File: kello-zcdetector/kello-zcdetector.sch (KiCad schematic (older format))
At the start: 8 parts, among them J1 Conn_01x02_Male, J2 Conn_01x02_Male, U1 LTV-817S

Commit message: joo
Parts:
- R1, R2, R3, R4: footprint Resistor_SMD:R_1206_3216Metric -> Resistor_SMD:R_0805_2012Metric
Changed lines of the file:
@@
 F 0 "R1" V 1893 3150 50  0000 C CNN
 F 1 "100k" V 1984 3150 50  0000 C CNN
-F 2 "Resistor_SMD:R_1206_3216Metric" V 2030 3150 50  0001 C CNN
+F 2 "Resistor_SMD:R_0805_2012Metric" V 2030 3150 50  0001 C CNN
 F 3 "~" H 2100 3150 50  0001 C CNN
 	1    2100 3150
@@
 F 0 "R2" V 1893 3500 50  0000 C CNN
 F 1 "100k" V 1984 3500 50  0000 C CNN
-F 2 "Resistor_SMD:R_1206_3216Metric" V 2030 3500 50  0001 C CNN
+F 2 "Resistor_SMD:R_0805_2012Metric" V 2030 3500 50  0001 C CNN
 F 3 "~" H 2100 3500 50  0001 C CNN
 	1    2100 3500
@@
 F 0 "R3" V 2393 3150 50  0000 C CNN
 F 1 "100k" V 2484 3150 50  0000 C CNN
-F 2 "Resistor_SMD:R_1206_3216Metric" V 2530 3150 50  0001 C CNN
+F 2 "Resistor_SMD:R_0805_2012Metric" V 2530 3150 50  0001 C CNN
 F 3 "~" H 2600 3150 50  0001 C CNN
 	1    2600 3150
@@
 F 0 "R4" V 2393 3500 50  0000 C CNN
 F 1 "100k" V 2484 3500 50  0000 C CNN
-F 2 "Resistor_SMD:R_1206_3216Metric" V 2530 3500 50  0001 C CNN
+F 2 "Resistor_SMD:R_0805_2012Metric" V 2530 3500 50  0001 C CNN
 F 3 "~" H 2600 3500 50  0001 C CNN
 	1    2600 3500

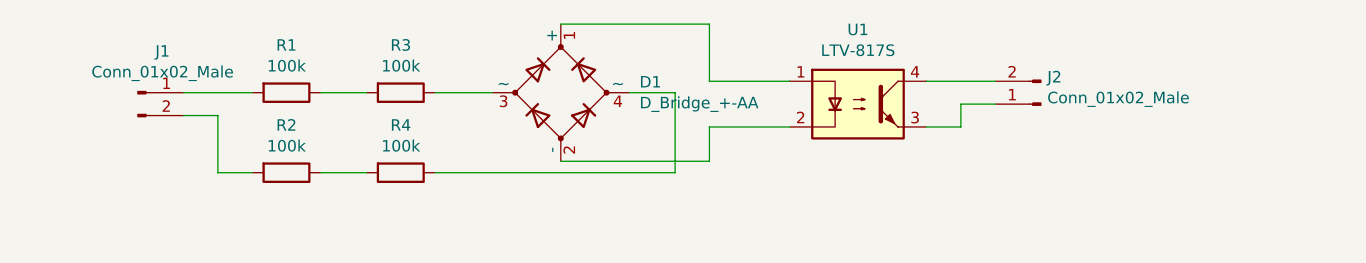
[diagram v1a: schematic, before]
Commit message: joo
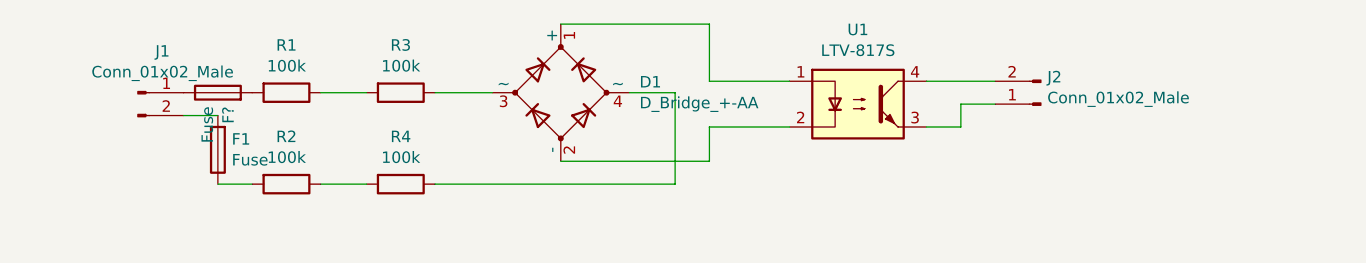
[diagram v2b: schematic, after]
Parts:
- added F1, F?: Fuse, Fuse:Fuse_10mmx3mm, symbol Device:Fuse
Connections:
- net at R1.2: now also F?.2; no longer J1.1 (Pin_1)
- net at R2.2: now also F1.1; no longer J1.2 (Pin_2)
- new net: F1.2, J1.2 (Pin_2)
- new net: F?.1, J1.1 (Pin_1)
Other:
- moved on the sheet: R2, R4
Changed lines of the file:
@@
 L Device:R R2
 U 1 1 5E892730
-P 2100 3500
-F 0 "R2" V 1893 3500 50  0000 C CNN
-F 1 "100k" V 1984 3500 50  0000 C CNN
-F 2 "Resistor_SMD:R_0805_2012Metric" V 2030 3500 50  0001 C CNN
-F 3 "~" H 2100 3500 50  0001 C CNN
-	1    2100 3500
+P 2100 3550
+F 0 "R2" V 1893 3550 50  0000 C CNN
+F 1 "100k" V 1984 3550 50  0000 C CNN
+F 2 "Resistor_SMD:R_0805_2012Metric" V 2030 3550 50  0001 C CNN
+F 3 "~" H 2100 3550 50  0001 C CNN
+	1    2100 3550
 	0    1    1    0
 $EndComp
@@
 L Device:R R4
 U 1 1 5E8929D6
-P 2600 3500
-F 0 "R4" V 2393 3500 50  0000 C CNN
-F 1 "100k" V 2484 3500 50  0000 C CNN
-F 2 "Resistor_SMD:R_0805_2012Metric" V 2530 3500 50  0001 C CNN
-F 3 "~" H 2600 3500 50  0001 C CNN
-	1    2600 3500
+P 2600 3550
+F 0 "R4" V 2393 3550 50  0000 C CNN
+F 1 "100k" V 2484 3550 50  0000 C CNN
+F 2 "Resistor_SMD:R_0805_2012Metric" V 2530 3550 50  0001 C CNN
+F 3 "~" H 2600 3550 50  0001 C CNN
+	1    2600 3550
 	0    1    1    0
 $EndComp
@@
 $EndComp
 Wire Wire Line
-	1650 3150 1950 3150
-Wire Wire Line
 	1650 3250 1800 3250
 Wire Wire Line
-	1800 3250 1800 3500
-Wire Wire Line
-	1800 3500 1950 3500
-Wire Wire Line
-	2250 3500 2450 3500
+	2250 3550 2450 3550
 Wire Wire Line
 	2250 3150 2450 3150
@@
 	3000 3150 2750 3150
 Wire Wire Line
-	2750 3500 3800 3500
-Wire Wire Line
-	3800 3500 3800 3150
+	2750 3550 3800 3550
 Wire Wire Line
 	3800 3150 3600 3150
@@
 Wire Wire Line
 	5050 3200 5200 3200
+$Comp
+L Device:Fuse F1
+U 1 1 5E4EBF45
+P 1800 3400
+F 0 "F1" H 1740 3354 50  0000 R CNN
+F 1 "Fuse" H 1740 3445 50  0000 R CNN
+F 2 "Fuse:Fuse_10mmx3mm" V 1730 3400 50  0001 C CNN
+F 3 "~" H 1800 3400 50  0001 C CNN
+	1    1800 3400
+	-1   0    0    1
+$EndComp
+Wire Wire Line
+	3800 3150 3800 3550
+Wire Wire Line
+	1800 3550 1950 3550
+$Comp
+L Device:Fuse F?
+U 1 1 5EDDD343
+P 1800 3150
+F 0 "F?" H 1740 3104 50  0000 R CNN
+F 1 "Fuse" H 1740 3195 50  0000 R CNN
+F 2 "Fuse:Fuse_10mmx3mm" V 1730 3150 50  0001 C CNN
+F 3 "~" H 1800 3150 50  0001 C CNN
+	1    1800 3150
+	0    -1   -1   0
+$EndComp
 $EndSCHEMATC

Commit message: diodisillalla zcdet
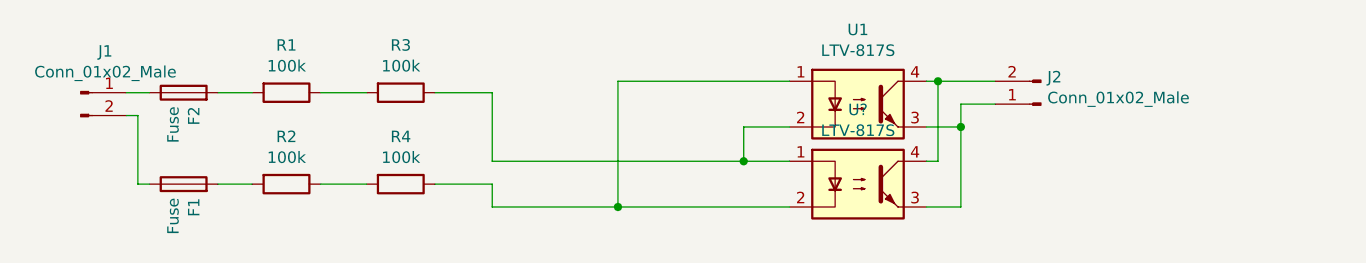
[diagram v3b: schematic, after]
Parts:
- removed D1: D_Bridge_+-AA, Diode_SMD:Diode_Bridge_Diotec_SO-DIL-Slim, symbol Device:D_Bridge_+-AA
- added U?: LTV-817S, Package_DIP:SMDIP-4_W9.53mm, symbol Isolator:LTV-817S
- gave numbers to parts that had none: 1
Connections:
- net at F1.1: now also J1.2 (Pin_2); no longer R2.2
- net at F1.2: now also R2.2; no longer J1.2 (Pin_2)
- net at R3.1: now also U1.2, U?.1
- net at R4.1: now also U1.1, U?.2
- net at J2.1 (Pin_1), U1.3: now also U?.3
- net at J2.2 (Pin_2), U1.4: now also U?.4
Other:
- moved on the sheet: F1, F2, J1
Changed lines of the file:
@@
 L Connector:Conn_01x02_Male J1
 U 1 1 5E892E28
-P 1450 3150
-F 0 "J1" H 1558 3331 50  0000 C CNN
-F 1 "Conn_01x02_Male" H 1558 3240 50  0000 C CNN
-F 2 "Connector_PinHeader_2.54mm:PinHeader_1x02_P2.54mm_Vertical" H 1450 3150 50  0001 C CNN
-F 3 "~" H 1450 3150 50  0001 C CNN
-	1    1450 3150
+P 1200 3150
+F 0 "J1" H 1308 3331 50  0000 C CNN
+F 1 "Conn_01x02_Male" H 1308 3240 50  0000 C CNN
+F 2 "Connector_PinHeader_2.54mm:PinHeader_1x02_P2.54mm_Vertical" H 1200 3150 50  0001 C CNN
+F 3 "~" H 1200 3150 50  0001 C CNN
+	1    1200 3150
 	1    0    0    -1
 $EndComp
-Wire Wire Line
-	1650 3250 1800 3250
 Wire Wire Line
 	2250 3550 2450 3550
 Wire Wire Line
 	2250 3150 2450 3150
-$Comp
-L Device:D_Bridge_+-AA D1
-U 1 1 5E893821
-P 3300 3150
-F 0 "D1" V 3346 2806 50  0000 R CNN
-F 1 "D_Bridge_+-AA" V 3255 2806 50  0000 R CNN
-F 2 "Diode_SMD:Diode_Bridge_Diotec_SO-DIL-Slim" H 3300 3150 50  0001 C CNN
-F 3 "~" H 3300 3150 50  0001 C CNN
-	1    3300 3150
-	0    -1   -1   0
-$EndComp
 Wire Wire Line
 	3000 3150 2750 3150
-Wire Wire Line
-	2750 3550 3800 3550
-Wire Wire Line
-	3800 3150 3600 3150
 $Comp
 L Isolator:LTV-817S U1
@@
 	1    0    0    -1
 $EndComp
-Wire Wire Line
-	4300 3100 3950 3100
-Wire Wire Line
-	3950 3100 3950 2850
-Wire Wire Line
-	3950 2850 3300 2850
-Wire Wire Line
-	3300 3450 3950 3450
-Wire Wire Line
-	3950 3450 3950 3300
-Wire Wire Line
-	3950 3300 4300 3300
 $Comp
 L Connector:Conn_01x02_Male J2
@@
 $EndComp
 Wire Wire Line
-	5200 3100 4900 3100
+	5200 3100 4950 3100
 Wire Wire Line
 	5050 3200 5050 3300
@@
 L Device:Fuse F1
 U 1 1 5E4EBF45
-P 1800 3400
-F 0 "F1" H 1740 3354 50  0000 R CNN
-F 1 "Fuse" H 1740 3445 50  0000 R CNN
-F 2 "Fuse:Fuse_10mmx3mm" V 1730 3400 50  0001 C CNN
-F 3 "~" H 1800 3400 50  0001 C CNN
-	1    1800 3400
-	-1   0    0    1
+P 1650 3550
+F 0 "F1" H 1590 3504 50  0000 R CNN
+F 1 "Fuse" H 1590 3595 50  0000 R CNN
+F 2 "Fuse:Fuse_10mmx3mm" V 1580 3550 50  0001 C CNN
+F 3 "~" H 1650 3550 50  0001 C CNN
+	1    1650 3550
+	0    -1   -1   0
 $EndComp
-Wire Wire Line
-	3800 3150 3800 3550
 Wire Wire Line
 	1800 3550 1950 3550
 $Comp
-L Device:Fuse F?
+L Device:Fuse F2
 U 1 1 5EDDD343
-P 1800 3150
-F 0 "F?" H 1740 3104 50  0000 R CNN
-F 1 "Fuse" H 1740 3195 50  0000 R CNN
-F 2 "Fuse:Fuse_10mmx3mm" V 1730 3150 50  0001 C CNN
-F 3 "~" H 1800 3150 50  0001 C CNN
-	1    1800 3150
+P 1650 3150
+F 0 "F2" H 1590 3104 50  0000 R CNN
+F 1 "Fuse" H 1590 3195 50  0000 R CNN
+F 2 "Fuse:Fuse_10mmx3mm" V 1580 3150 50  0001 C CNN
+F 3 "~" H 1650 3150 50  0001 C CNN
+	1    1650 3150
 	0    -1   -1   0
 $EndComp
+$Comp
+L Isolator:LTV-817S U?
+U 1 1 5EDE879D
+P 4600 3550
+F 0 "U?" H 4600 3875 50  0000 C CNN
+F 1 "LTV-817S" H 4600 3784 50  0000 C CNN
+F 2 "Package_DIP:SMDIP-4_W9.53mm" H 4600 3250 50  0001 C CNN
+F 3 "http://www.us.liteon.com/downloads/LTV-817-827-847.PDF" H 4250 3850 50  0001 C CNN
+	1    4600 3550
+	1    0    0    -1
+$EndComp
+Wire Wire Line
+	4900 3450 4950 3450
+Wire Wire Line
+	4950 3450 4950 3100
+Connection ~ 4950 3100
+Wire Wire Line
+	4950 3100 4900 3100
+Wire Wire Line
+	5050 3300 5050 3650
+Wire Wire Line
+	5050 3650 4900 3650
+Connection ~ 5050 3300
+Wire Wire Line
+	2750 3550 3000 3550
+Wire Wire Line
+	3550 3650 4300 3650
+Wire Wire Line
+	4300 3100 3550 3100
+Wire Wire Line
+	4300 3300 4100 3300
+Wire Wire Line
+	4300 3450 4100 3450
+Wire Wire Line
+	4100 3450 4100 3300
+Wire Wire Line
+	1500 3150 1400 3150
+Wire Wire Line
+	1400 3250 1450 3250
+Wire Wire Line
+	1450 3250 1450 3550
+Wire Wire Line
+	1450 3550 1500 3550
+Wire Wire Line
+	1800 3150 1950 3150
+Wire Wire Line
+	4100 3450 3000 3450
+Connection ~ 4100 3450
+Wire Wire Line
+	3000 3150 3000 3450
+Wire Wire Line
+	3550 3650 3000 3650
+Wire Wire Line
+	3000 3650 3000 3550
+Connection ~ 3550 3650
+Wire Wire Line
+	3550 3100 3550 3650
 $EndSCHEMATC

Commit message: jawohl
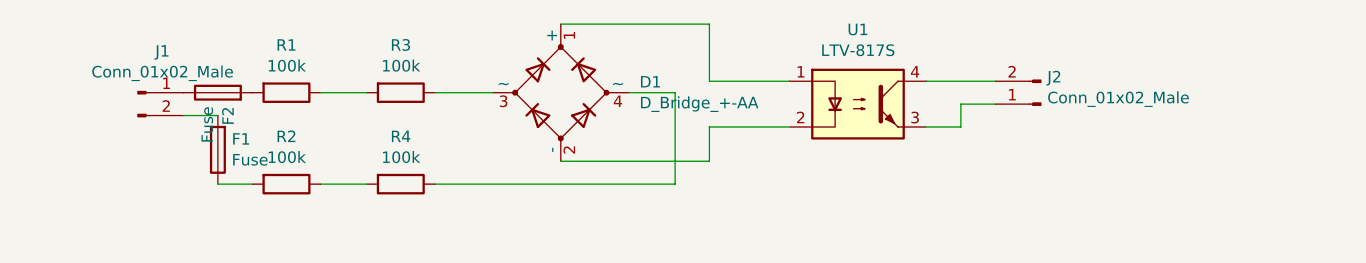
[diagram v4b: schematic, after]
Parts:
- removed U?: LTV-817S, Package_DIP:SMDIP-4_W9.53mm, symbol Isolator:LTV-817S
- added D1: D_Bridge_+-AA, Diode_SMD:Diode_Bridge_Diotec_SO-DIL-Slim, symbol Device:D_Bridge_+-AA
- J1: footprint Connector_PinHeader_2.54mm:PinHeader_1x02_P2.54mm_Vertical -> Connector_PinHeader_2.54mm:AC_connector
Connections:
- net at F1.1: now also R2.2; no longer J1.2 (Pin_2)
- net at F1.2: now also J1.2 (Pin_2); no longer R2.2
- net at R3.1: now also D1.3 (~~); no longer U1.2
- net at R4.1: now also D1.4 (~~); no longer U1.1
- new net: D1.1 (+), U1.1
- new net: D1.2 (-), U1.2
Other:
- moved on the sheet: F1, F2, J1
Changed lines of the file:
@@
 	0    1    1    0
-$EndComp
-$Comp
-L Connector:Conn_01x02_Male J1
-U 1 1 5E892E28
-P 1200 3150
-F 0 "J1" H 1308 3331 50  0000 C CNN
-F 1 "Conn_01x02_Male" H 1308 3240 50  0000 C CNN
-F 2 "Connector_PinHeader_2.54mm:PinHeader_1x02_P2.54mm_Vertical" H 1200 3150 50  0001 C CNN
-F 3 "~" H 1200 3150 50  0001 C CNN
-	1    1200 3150
-	1    0    0    -1
 $EndComp
 Wire Wire Line
@@
 Wire Wire Line
 	2250 3150 2450 3150
-Wire Wire Line
-	3000 3150 2750 3150
 $Comp
 L Isolator:LTV-817S U1
@@
 $EndComp
 Wire Wire Line
-	5200 3100 4950 3100
-Wire Wire Line
 	5050 3200 5050 3300
 Wire Wire Line
@@
 Wire Wire Line
 	5050 3200 5200 3200
+Wire Wire Line
+	1800 3550 1950 3550
+Wire Wire Line
+	1650 3250 1800 3250
+$Comp
+L Device:Fuse F2
+U 1 1 5EDDD343
+P 1800 3150
+F 0 "F2" H 1740 3104 50  0000 R CNN
+F 1 "Fuse" H 1740 3195 50  0000 R CNN
+F 2 "Fuse:Fuse_10mmx3mm" V 1730 3150 50  0001 C CNN
+F 3 "~" H 1800 3150 50  0001 C CNN
+	1    1800 3150
+	0    -1   -1   0
+$EndComp
+$Comp
+L Connector:Conn_01x02_Male J1
+U 1 1 5E892E28
+P 1450 3150
+F 0 "J1" H 1558 3331 50  0000 C CNN
+F 1 "Conn_01x02_Male" H 1558 3240 50  0000 C CNN
+F 2 "Connector_PinHeader_2.54mm:AC_connector" H 1450 3150 50  0001 C CNN
+F 3 "~" H 1450 3150 50  0001 C CNN
+	1    1450 3150
+	1    0    0    -1
+$EndComp
 $Comp
 L Device:Fuse F1
 U 1 1 5E4EBF45
-P 1650 3550
-F 0 "F1" H 1590 3504 50  0000 R CNN
-F 1 "Fuse" H 1590 3595 50  0000 R CNN
-F 2 "Fuse:Fuse_10mmx3mm" V 1580 3550 50  0001 C CNN
-F 3 "~" H 1650 3550 50  0001 C CNN
-	1    1650 3550
+P 1800 3400
+F 0 "F1" H 1740 3354 50  0000 R CNN
+F 1 "Fuse" H 1740 3445 50  0000 R CNN
+F 2 "Fuse:Fuse_10mmx3mm" V 1730 3400 50  0001 C CNN
+F 3 "~" H 1800 3400 50  0001 C CNN
+	1    1800 3400
+	-1   0    0    1
+$EndComp
+Wire Wire Line
+	3950 3300 4300 3300
+Wire Wire Line
+	3950 3450 3950 3300
+Wire Wire Line
+	3300 3450 3950 3450
+Wire Wire Line
+	3950 2850 3300 2850
+Wire Wire Line
+	3950 3100 3950 2850
+Wire Wire Line
+	4300 3100 3950 3100
+Wire Wire Line
+	5200 3100 4900 3100
+$Comp
+L Device:D_Bridge_+-AA D1
+U 1 1 5E893821
+P 3300 3150
+F 0 "D1" V 3346 2806 50  0000 R CNN
+F 1 "D_Bridge_+-AA" V 3255 2806 50  0000 R CNN
+F 2 "Diode_SMD:Diode_Bridge_Diotec_SO-DIL-Slim" H 3300 3150 50  0001 C CNN
+F 3 "~" H 3300 3150 50  0001 C CNN
+	1    3300 3150
 	0    -1   -1   0
 $EndComp
 Wire Wire Line
-	1800 3550 1950 3550
-$Comp
-L Device:Fuse F2
-U 1 1 5EDDD343
-P 1650 3150
-F 0 "F2" H 1590 3104 50  0000 R CNN
-F 1 "Fuse" H 1590 3195 50  0000 R CNN
-F 2 "Fuse:Fuse_10mmx3mm" V 1580 3150 50  0001 C CNN
-F 3 "~" H 1650 3150 50  0001 C CNN
-	1    1650 3150
-	0    -1   -1   0
-$EndComp
-$Comp
-L Isolator:LTV-817S U?
-U 1 1 5EDE879D
-P 4600 3550
-F 0 "U?" H 4600 3875 50  0000 C CNN
-F 1 "LTV-817S" H 4600 3784 50  0000 C CNN
-F 2 "Package_DIP:SMDIP-4_W9.53mm" H 4600 3250 50  0001 C CNN
-F 3 "http://www.us.liteon.com/downloads/LTV-817-827-847.PDF" H 4250 3850 50  0001 C CNN
-	1    4600 3550
-	1    0    0    -1
-$EndComp
+	3800 3150 3800 3550
 Wire Wire Line
-	4900 3450 4950 3450
+	2750 3550 3800 3550
 Wire Wire Line
-	4950 3450 4950 3100
-Connection ~ 4950 3100
+	3800 3150 3600 3150
 Wire Wire Line
-	4950 3100 4900 3100
-Wire Wire Line
-	5050 3300 5050 3650
-Wire Wire Line
-	5050 3650 4900 3650
-Connection ~ 5050 3300
-Wire Wire Line
-	2750 3550 3000 3550
-Wire Wire Line
-	3550 3650 4300 3650
-Wire Wire Line
-	4300 3100 3550 3100
-Wire Wire Line
-	4300 3300 4100 3300
-Wire Wire Line
-	4300 3450 4100 3450
-Wire Wire Line
-	4100 3450 4100 3300
-Wire Wire Line
-	1500 3150 1400 3150
-Wire Wire Line
-	1400 3250 1450 3250
-Wire Wire Line
-	1450 3250 1450 3550
-Wire Wire Line
-	1450 3550 1500 3550
-Wire Wire Line
-	1800 3150 1950 3150
-Wire Wire Line
-	4100 3450 3000 3450
-Connection ~ 4100 3450
-Wire Wire Line
-	3000 3150 3000 3450
-Wire Wire Line
-	3550 3650 3000 3650
-Wire Wire Line
-	3000 3650 3000 3550
-Connection ~ 3550 3650
-Wire Wire Line
-	3550 3100 3550 3650
+	3000 3150 2750 3150
 $EndSCHEMATC

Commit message: joo
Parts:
- added R5: 47k, Resistor_SMD:R_0805_2012Metric, symbol Device:R
- J2: footprint Connector_PinHeader_2.54mm:PinHeader_1x02_P2.54mm_Vertical -> Connector_PinHeader_2.54mm:PinHeader_1x03_P2.54mm_Vertical; symbol Connector:Conn_01x02_Male -> Connector:Conn_01x03_Male
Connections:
- net at F1.2: now also J1.1 (Pin_1); no longer J1.2 (Pin_2)
- net at R1.2: now also F2.1; no longer F2.2
- net at J2.2 (Pin_2), U1.4: now also R5.1
- new net: J2.3 (Pin_3), R5.2
- new net: F2.2, J1.2 (Pin_2)
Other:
- moved on the sheet: F2, J1
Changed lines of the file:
@@
 	1    0    0    -1
-$EndComp
-$Comp
-L Connector:Conn_01x02_Male J2
-U 1 1 5E895CD5
-P 5400 3200
-F 0 "J2" H 5372 3082 50  0000 R CNN
-F 1 "Conn_01x02_Male" H 5372 3173 50  0000 R CNN
-F 2 "Connector_PinHeader_2.54mm:PinHeader_1x02_P2.54mm_Vertical" H 5400 3200 50  0001 C CNN
-F 3 "~" H 5400 3200 50  0001 C CNN
-	1    5400 3200
-	-1   0    0    1
 $EndComp
 Wire Wire Line
@@
 Wire Wire Line
 	5050 3300 4900 3300
-Wire Wire Line
-	5050 3200 5200 3200
-Wire Wire Line
-	1800 3550 1950 3550
-Wire Wire Line
-	1650 3250 1800 3250
 $Comp
 L Device:Fuse F2
 U 1 1 5EDDD343
-P 1800 3150
-F 0 "F2" H 1740 3104 50  0000 R CNN
-F 1 "Fuse" H 1740 3195 50  0000 R CNN
-F 2 "Fuse:Fuse_10mmx3mm" V 1730 3150 50  0001 C CNN
-F 3 "~" H 1800 3150 50  0001 C CNN
-	1    1800 3150
-	0    -1   -1   0
+P 1600 3250
+F 0 "F2" H 1540 3204 50  0000 R CNN
+F 1 "Fuse" H 1540 3295 50  0000 R CNN
+F 2 "Fuse:Fuse_10mmx3mm" V 1530 3250 50  0001 C CNN
+F 3 "~" H 1600 3250 50  0001 C CNN
+	1    1600 3250
+	0    1    1    0
 $EndComp
 $Comp
 L Connector:Conn_01x02_Male J1
 U 1 1 5E892E28
-P 1450 3150
-F 0 "J1" H 1558 3331 50  0000 C CNN
-F 1 "Conn_01x02_Male" H 1558 3240 50  0000 C CNN
-F 2 "Connector_PinHeader_2.54mm:AC_connector" H 1450 3150 50  0001 C CNN
-F 3 "~" H 1450 3150 50  0001 C CNN
-	1    1450 3150
+P 1250 3150
+F 0 "J1" H 1358 3331 50  0000 C CNN
+F 1 "Conn_01x02_Male" H 1358 3240 50  0000 C CNN
+F 2 "Connector_PinHeader_2.54mm:AC_connector" H 1250 3150 50  0001 C CNN
+F 3 "~" H 1250 3150 50  0001 C CNN
+	1    1250 3150
 	1    0    0    -1
 $EndComp
@@
 Wire Wire Line
 	4300 3100 3950 3100
-Wire Wire Line
-	5200 3100 4900 3100
 $Comp
 L Device:D_Bridge_+-AA D1
@@
 Wire Wire Line
 	3000 3150 2750 3150
+$Comp
+L Device:R R5
+U 1 1 5E5E3A5F
+P 5350 3000
+F 0 "R5" V 5143 3000 50  0000 C CNN
+F 1 "47k" V 5234 3000 50  0000 C CNN
+F 2 "Resistor_SMD:R_0805_2012Metric" V 5280 3000 50  0001 C CNN
+F 3 "~" H 5350 3000 50  0001 C CNN
+	1    5350 3000
+	0    -1   -1   0
+$EndComp
+$Comp
+L Connector:Conn_01x03_Male J2
+U 1 1 5E895CD5
+P 5950 3100
+F 0 "J2" H 5922 2982 50  0000 R CNN
+F 1 "Conn_01x02_Male" H 5922 3073 50  0000 R CNN
+F 2 "Connector_PinHeader_2.54mm:PinHeader_1x03_P2.54mm_Vertical" H 5950 3100 50  0001 C CNN
+F 3 "~" H 5950 3100 50  0001 C CNN
+	1    5950 3100
+	-1   0    0    1
+$EndComp
+Wire Wire Line
+	5050 3200 5750 3200
+Wire Wire Line
+	4900 3100 5100 3100
+Wire Wire Line
+	5750 3000 5500 3000
+Wire Wire Line
+	5200 3000 5100 3000
+Wire Wire Line
+	5100 3000 5100 3100
+Connection ~ 5100 3100
+Wire Wire Line
+	5100 3100 5750 3100
+Wire Wire Line
+	1800 3550 1950 3550
+Wire Wire Line
+	1800 3250 1800 3150
+Wire Wire Line
+	1800 3150 1450 3150
+Wire Wire Line
+	1750 3250 1750 3200
+Wire Wire Line
+	1750 3200 1950 3200
+Wire Wire Line
+	1950 3200 1950 3150
 $EndSCHEMATC
